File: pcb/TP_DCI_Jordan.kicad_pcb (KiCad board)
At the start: 2 copper layers, 52 x 30 mm, 19 parts, among them J1 MICRO, J2 Display, SW1 SW_DIP_x03, U1 PCF8574

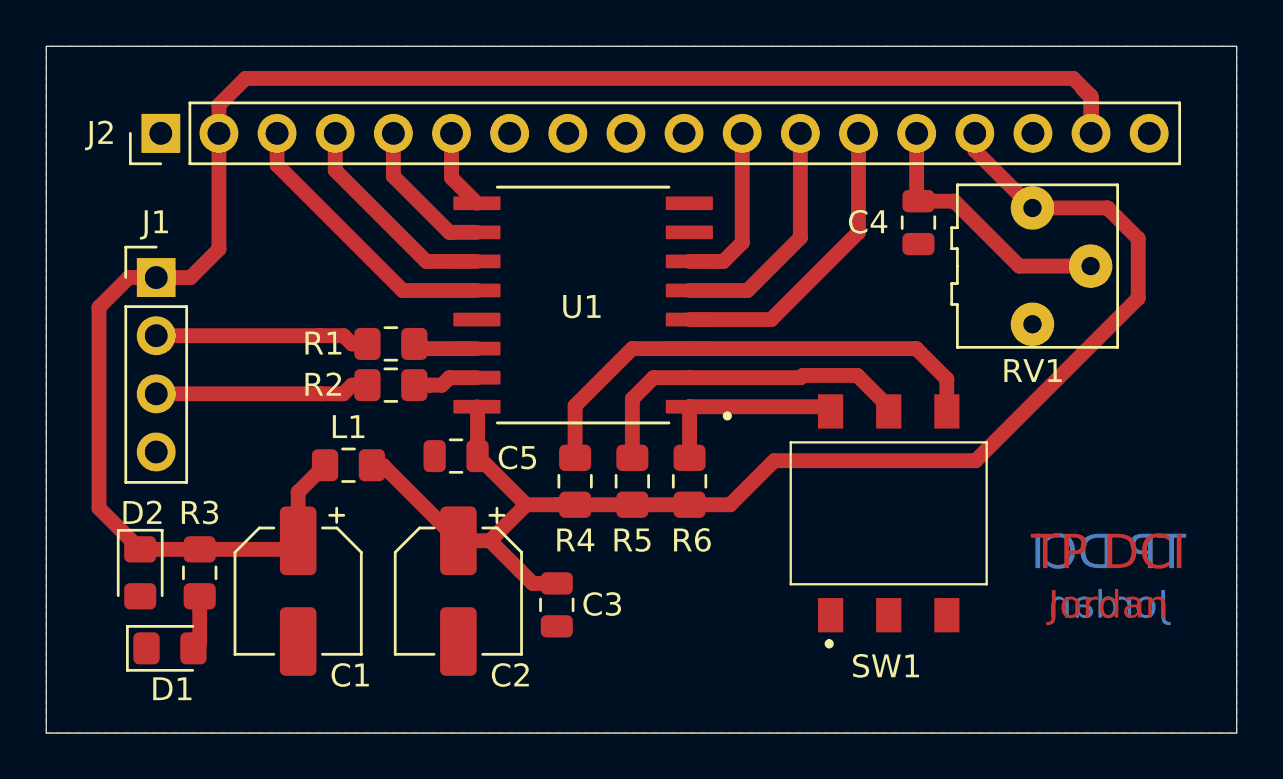
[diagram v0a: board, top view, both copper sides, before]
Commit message: carpetas doc e info ok
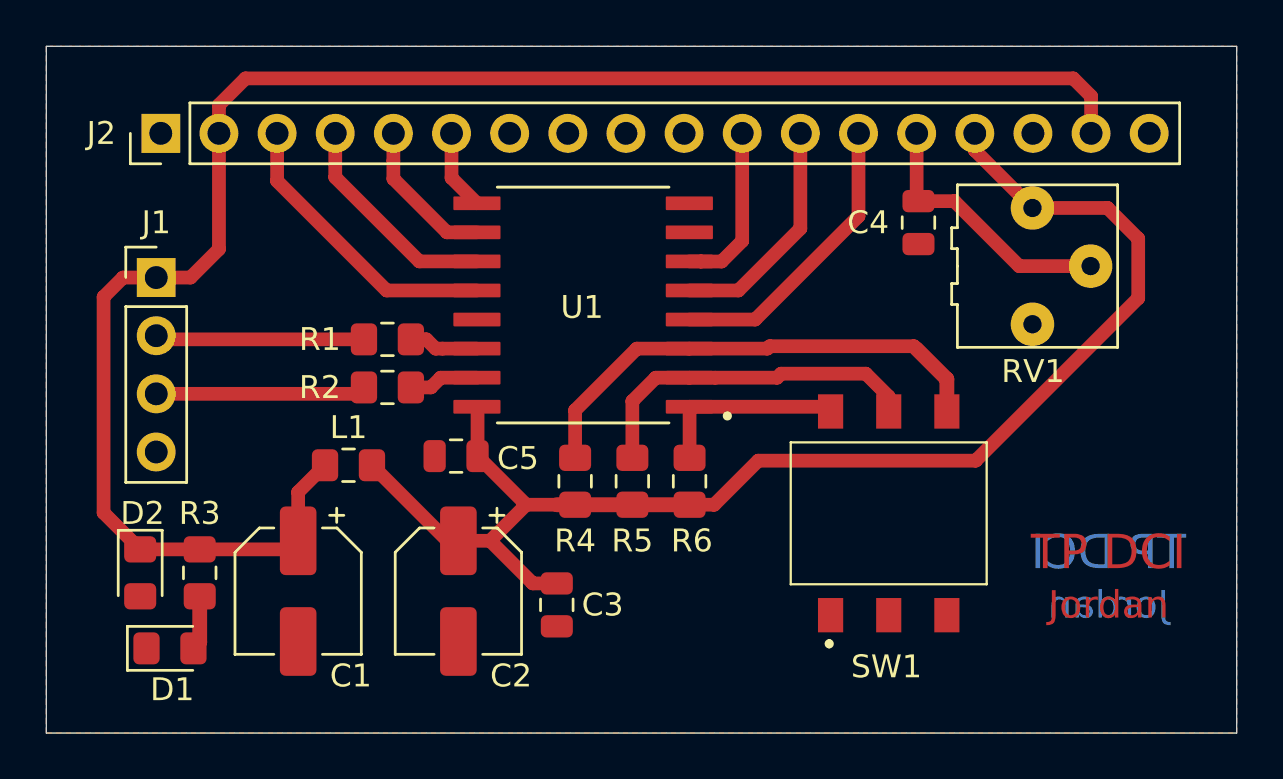
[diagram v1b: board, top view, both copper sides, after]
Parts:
- moved R1 0.25 mm to (96.3, 123.2)
- moved R2 0.18 mm to (96.3, 125.3)
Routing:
- net /Vin: track 77.5 -> 75.4 mm
- net Net-(R4-Pad1): track 21.5 -> 23.4 mm
- net Net-(R2-Pad2): track 3.58 -> 3.06 mm
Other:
- net class Default: clearance 0.5 -> 0.6; trace_width 0.65 -> 0.6
- rule trace_clearance: 0.5 -> 0.6
- rule trace_min: 0.2 -> 0.6
